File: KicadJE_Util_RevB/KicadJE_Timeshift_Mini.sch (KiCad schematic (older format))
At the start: 60 parts, among them J301 In3.1, J302 Out3.1, J303 Out3.2, P301 HEADER_2x5_Doepfer, U301 TL072, U302 TL072

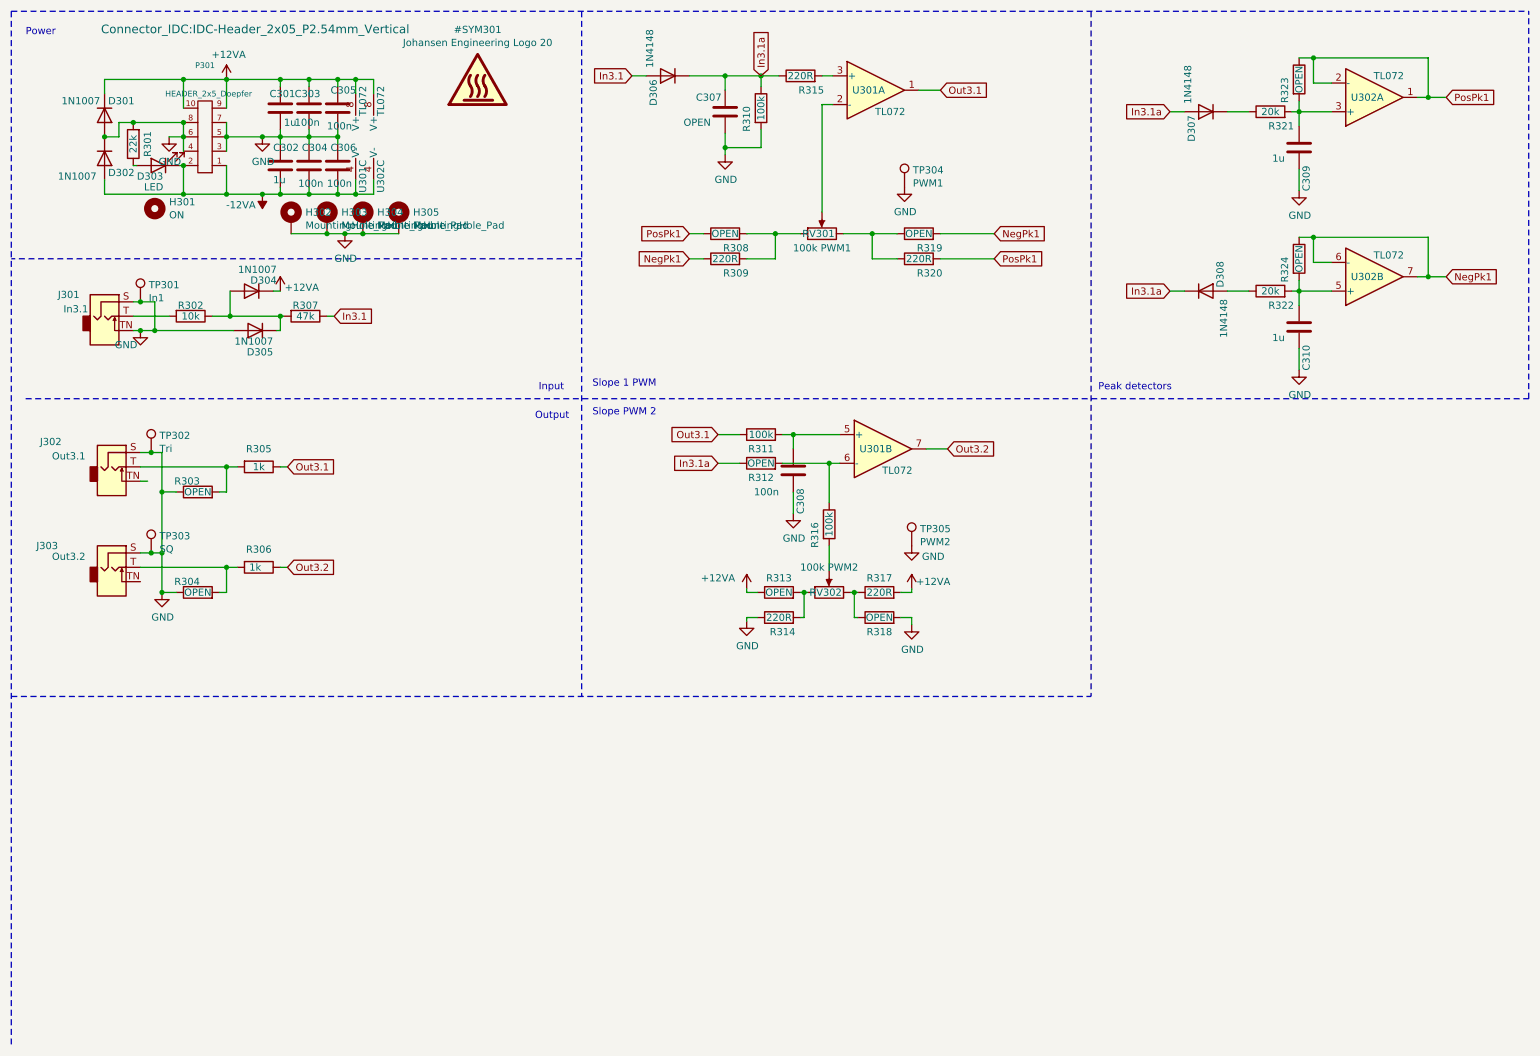
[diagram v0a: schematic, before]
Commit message: Update KicadJE_Timeshift_Mini.sch
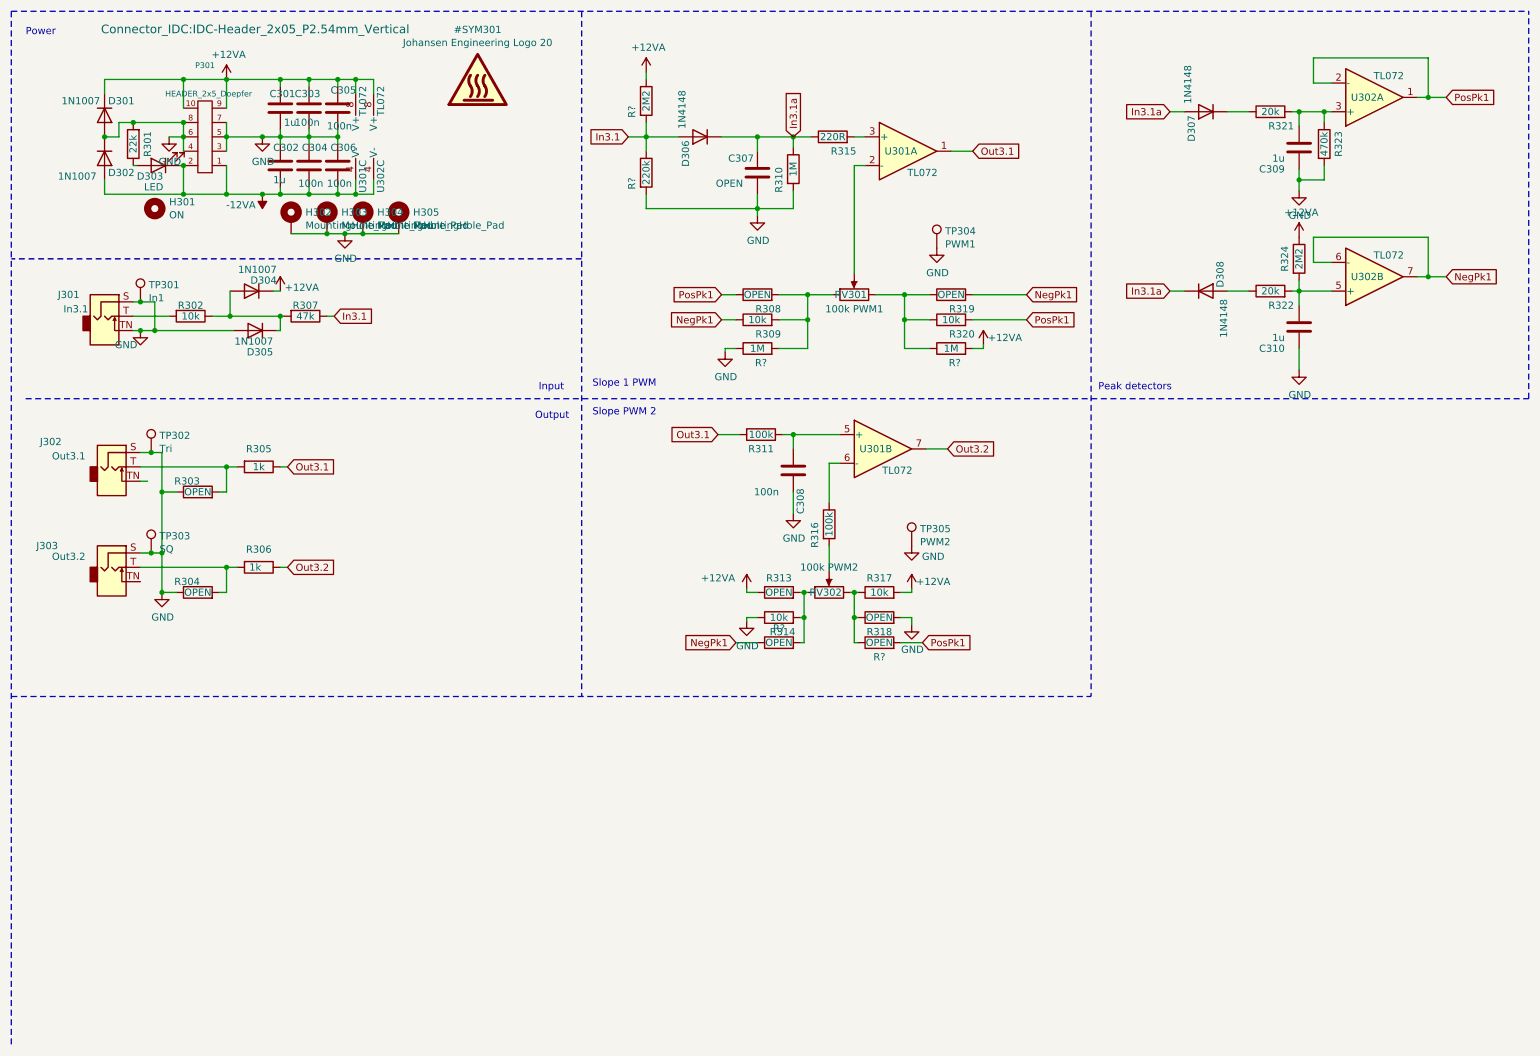
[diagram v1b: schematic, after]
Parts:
- removed R312: OPEN, Resistor_SMD:R_0805_2012Metric_Pad1.15x1.40mm_HandSolder, symbol Device:R
- added R?: 220k, Resistor_SMD:R_0805_2012Metric_Pad1.15x1.40mm_HandSolder, symbol Device:R
- added R?: 2M2, Resistor_SMD:R_0805_2012Metric_Pad1.15x1.40mm_HandSolder, symbol Device:R
- added R? (x2): 1M, Resistor_SMD:R_0805_2012Metric_Pad1.15x1.40mm_HandSolder, symbol Device:R
- added R? (x2): OPEN, Resistor_SMD:R_0805_2012Metric_Pad1.15x1.40mm_HandSolder, symbol Device:R
- R309, R314, R317, R320: value 220R -> 10k
- R310: value 100k -> 1M
- R323: value OPEN -> 470k
- R324: value OPEN -> 2M2
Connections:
- net +12VA: now also R324.1, R?.1, R?.2
- net GND: now also R323.2, R?.1, R?.2
- net In3.1: now also R?.1, R?.2
- net NegPk1: now also R?.1; no longer R324.1
- net PosPk1: now also R?.2; no longer R323.1
- net at R308.2, R309.2, RV301.1: now also R?.2
- net at R319.1, R320.1, RV301.3: now also R?.1
- net at C309.2, R321.2, U302.3 (+): now also R323.1; no longer R323.2
- net at R313.2, R314.2, RV302.1: now also R?.2
- net at R317.1, R318.1, RV302.3: now also R?.1
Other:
- moved on the sheet: C307, D306, R308, R309, R310, R315, R319, R320, R323, RV301, TP304, U301A

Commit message: Update KicadJE_Timeshift_Mini.sch
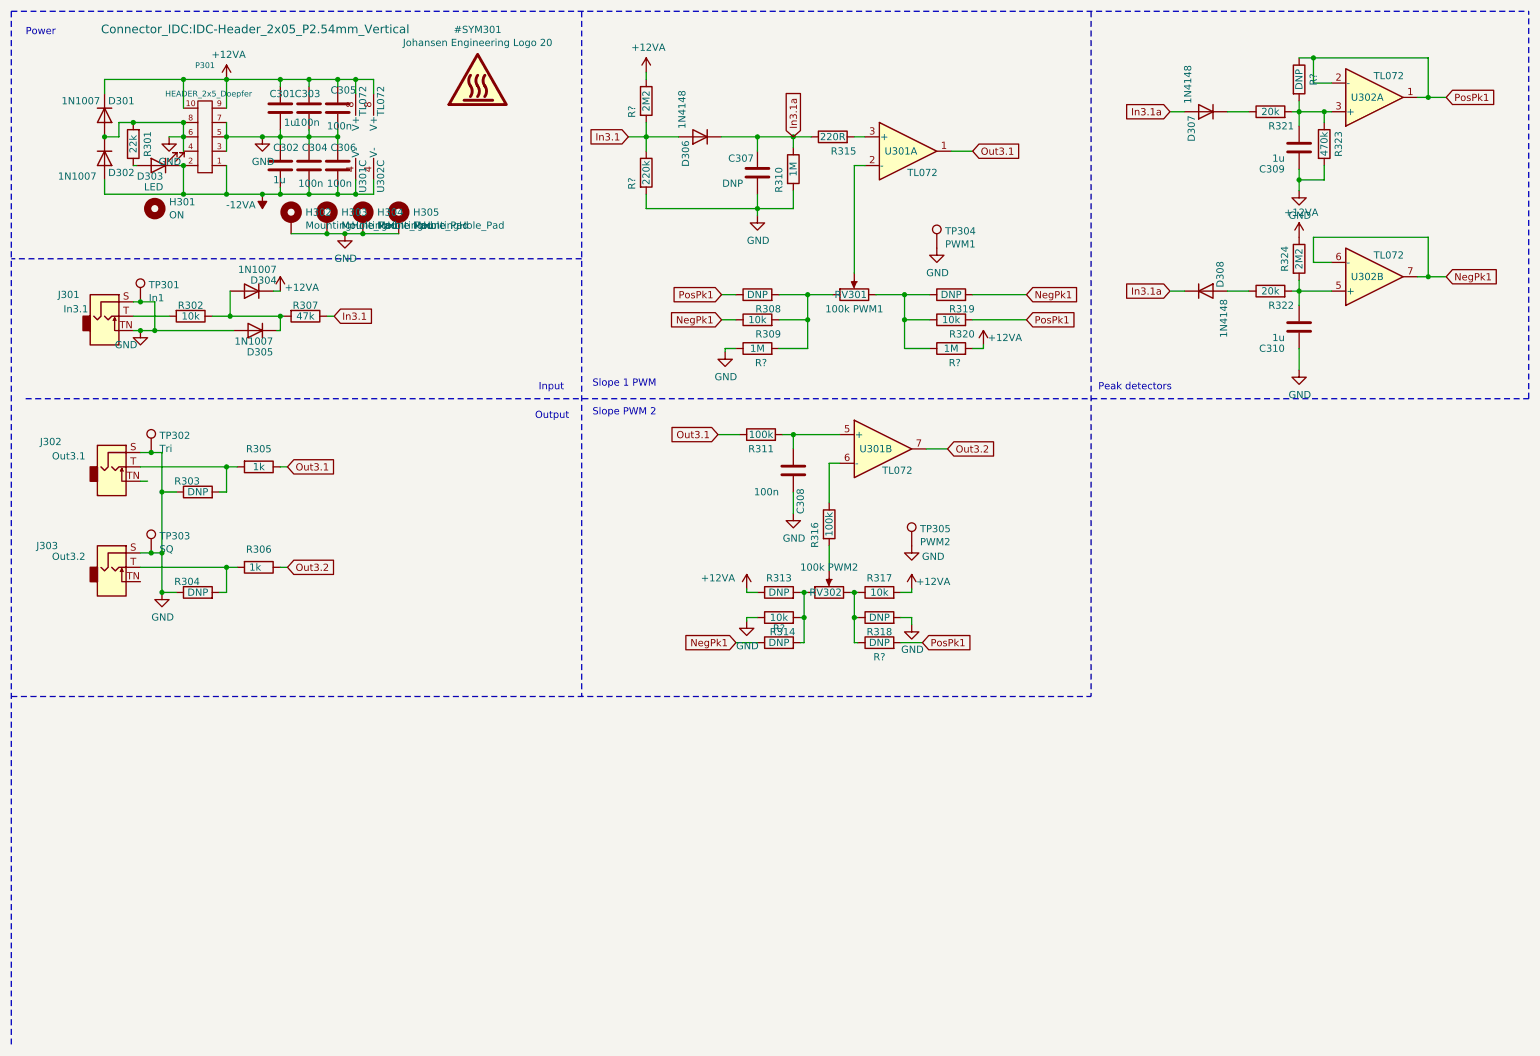
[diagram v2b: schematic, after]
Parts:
- added R?: DNP, Resistor_SMD:R_0805_2012Metric_Pad1.15x1.40mm_HandSolder, symbol Device:R
- C307, R303, R304, R308, R313, R318, R319, R? (x2): value OPEN -> DNP
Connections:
- net PosPk1: now also R?.1
- net at C309.2, R321.2, R323.1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: now also R?.2
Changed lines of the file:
@@
 AR Path="/5EFABE3E/5EFCD44F" Ref="R304"  Part="1"
 F 0 "R304" V 1900 4675 50  0000 C CNN
-F 1 "OPEN" V 1825 4600 50  0000 C CNN
+F 1 "DNP" V 1825 4600 50  0000 C CNN
 F 2 "Resistor_SMD:R_0805_2012Metric_Pad1.15x1.40mm_HandSolder" V 1755 4600 50  0001 C CNN
 F 3 "~" H 1825 4600 50  0001 C CNN
@@
 AR Path="/5EFABE3E/5EFCD52A" Ref="R303"  Part="1"
 F 0 "R303" V 1900 3975 50  0000 C CNN
-F 1 "OPEN" V 1825 3900 50  0000 C CNN
+F 1 "DNP" V 1825 3900 50  0000 C CNN
 F 2 "Resistor_SMD:R_0805_2012Metric_Pad1.15x1.40mm_HandSolder" V 1755 3900 50  0001 C CNN
 F 3 "~" H 1825 3900 50  0001 C CNN
@@
 AR Path="/5EFABE3E/5F001C3B" Ref="R308"  Part="1"
 F 0 "R308" V 5625 2450 50  0000 C CNN
-F 1 "OPEN" V 5725 2525 50  0000 C CNN
+F 1 "DNP" V 5725 2525 50  0000 C CNN
 F 2 "Resistor_SMD:R_0805_2012Metric_Pad1.15x1.40mm_HandSolder" V 5655 2525 50  0001 C CNN
 F 3 "~" H 5725 2525 50  0001 C CNN
@@
 AR Path="/5EFABE3E/5F001CA1" Ref="C307"  Part="1"
 F 0 "C307" H 5750 1575 50  0000 L CNN
-F 1 "OPEN" H 5825 1750 50  0000 L CNN
+F 1 "DNP" H 5825 1750 50  0000 L CNN
 F 2 "Capacitor_SMD:C_0805_2012Metric_Pad1.15x1.40mm_HandSolder" H 5763 1525 50  0001 C CNN
 F 3 "~" H 5725 1675 50  0001 C CNN
@@
 AR Path="/5EFABE3E/5F122A16" Ref="R319"  Part="1"
 F 0 "R319" V 6975 2450 50  0000 C CNN
-F 1 "OPEN" V 7075 2525 50  0000 C CNN
+F 1 "DNP" V 7075 2525 50  0000 C CNN
 F 2 "Resistor_SMD:R_0805_2012Metric_Pad1.15x1.40mm_HandSolder" V 7005 2525 50  0001 C CNN
 F 3 "~" H 7075 2525 50  0001 C CNN
@@
 AR Path="/5EFABE3E/5F1DE0C3" Ref="R313"  Part="1"
 F 0 "R313" V 5975 4600 50  0000 C CNN
-F 1 "OPEN" V 5875 4600 50  0000 C CNN
+F 1 "DNP" V 5875 4600 50  0000 C CNN
 F 2 "Resistor_SMD:R_0805_2012Metric_Pad1.15x1.40mm_HandSolder" V 5805 4600 50  0001 C CNN
 F 3 "~" H 5875 4600 50  0001 C CNN
@@
 AR Path="/5EFABE3E/5F1DE11A" Ref="R318"  Part="1"
 F 0 "R318" V 6475 4775 50  0000 C CNN
-F 1 "OPEN" V 6575 4775 50  0000 C CNN
+F 1 "DNP" V 6575 4775 50  0000 C CNN
 F 2 "Resistor_SMD:R_0805_2012Metric_Pad1.15x1.40mm_HandSolder" V 6505 4775 50  0001 C CNN
 F 3 "~" H 6575 4775 50  0001 C CNN
@@
 AR Path="/5EFABE3E/5EA9FF23" Ref="R?"  Part="1"
 F 0 "R?" V 6475 4950 50  0000 C CNN
-F 1 "OPEN" V 6575 4950 50  0000 C CNN
+F 1 "DNP" V 6575 4950 50  0000 C CNN
 F 2 "Resistor_SMD:R_0805_2012Metric_Pad1.15x1.40mm_HandSolder" V 6505 4950 50  0001 C CNN
 F 3 "~" H 6575 4950 50  0001 C CNN
@@
 AR Path="/5EFABE3E/5EAAADA4" Ref="R?"  Part="1"
 F 0 "R?" V 5975 4950 50  0000 C CNN
-F 1 "OPEN" V 5875 4950 50  0000 C CNN
+F 1 "DNP" V 5875 4950 50  0000 C CNN
 F 2 "Resistor_SMD:R_0805_2012Metric_Pad1.15x1.40mm_HandSolder" V 5805 4950 50  0001 C CNN
 F 3 "~" H 5875 4950 50  0001 C CNN
@@
 Wire Wire Line
 	5575 4950 5725 4950
+$Comp
+L Device:R R?
+U 1 1 5EB19454
+P 9500 1025
+AR Path="/5EB19454" Ref="R?"  Part="1"
+AR Path="/5C8C5FC0/5EB19454" Ref="R?"  Part="1"
+AR Path="/5CAAE8D3/5EB19454" Ref="R?"  Part="1"
+AR Path="/5E4B0DD9/5EB19454" Ref="R?"  Part="1"
+AR Path="/5E62ACA1/5EB19454" Ref="R?"  Part="1"
+AR Path="/5F49A670/5EB19454" Ref="R?"  Part="1"
+AR Path="/5FDBD837/5EB19454" Ref="R?"  Part="1"
+AR Path="/5EFABE3E/5EB19454" Ref="R?"  Part="1"
+F 0 "R?" V 9600 1025 50  0000 C CNN
+F 1 "DNP" V 9500 1025 50  0000 C CNN
+F 2 "Resistor_SMD:R_0805_2012Metric_Pad1.15x1.40mm_HandSolder" V 9430 1025 50  0001 C CNN
+F 3 "~" H 9500 1025 50  0001 C CNN
+	1    9500 1025
+	1    0    0    -1
+$EndComp
+Wire Wire Line
+	9500 1250 9500 1175
+Connection ~ 9600 875
+Wire Wire Line
+	9500 875  9600 875
 $EndSCHEMATC

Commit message: attempt to go to Kicad 7
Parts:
- P301: symbol Eurorack:HEADER_2x5_Doepfer -> KicadJE_Util-rescue:HEADER_2x5_Doepfer-Eurorack
- RV301, RV302: symbol Envelope-cache-2018-08-04-13-00-04:POT -> KicadJE_Util-rescue:POT-Envelope-cache-2018-08-04-13-00-04
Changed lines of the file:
@@
 $EndComp
 $Comp
-L Envelope-cache-2018-08-04-13-00-04:GND #PWR?
+L KicadJE_Util-rescue:GND-Envelope-cache-2018-08-04-13-00-04 #PWR?
 U 1 1 5EFCD382
 P 1575 4600
@@
 $EndComp
 $Comp
-L Eurorack:HEADER_2x5_Doepfer P?
+L KicadJE_Util-rescue:HEADER_2x5_Doepfer-Eurorack P?
 U 1 1 5EFCD3D2
 P 1875 1425
@@
 	2400 1075 2400 1025
 $Comp
-L Envelope-cache-2018-08-04-13-00-04:GND #PWR?
+L KicadJE_Util-rescue:GND-Envelope-cache-2018-08-04-13-00-04 #PWR?
 U 1 1 5EFCD408
 P 2275 1425
@@
 $EndComp
 $Comp
-L Envelope-cache-2018-08-04-13-00-04:GND #PWR?
+L KicadJE_Util-rescue:GND-Envelope-cache-2018-08-04-13-00-04 #PWR?
 U 1 1 5EFCD41A
 P 1625 1425
@@
 Connection ~ 2975 2100
 $Comp
-L Envelope-cache-2018-08-04-13-00-04:GND #PWR?
+L KicadJE_Util-rescue:GND-Envelope-cache-2018-08-04-13-00-04 #PWR?
 U 1 1 5EFCD514
 P 2850 2100
@@
 	1425 2575 1375 2575
 $Comp
-L Envelope-cache-2018-08-04-13-00-04:GND #PWR?
+L KicadJE_Util-rescue:GND-Envelope-cache-2018-08-04-13-00-04 #PWR?
 U 1 1 5F001BB2
 P 1425 2775
@@
 $EndComp
 $Comp
-L Envelope-cache-2018-08-04-13-00-04:POT RV?
+L KicadJE_Util-rescue:POT-Envelope-cache-2018-08-04-13-00-04 RV?
 U 1 1 5F001C35
 P 6400 2525
@@
 $EndComp
 $Comp
-L Envelope-cache-2018-08-04-13-00-04:GND #PWR?
+L KicadJE_Util-rescue:GND-Envelope-cache-2018-08-04-13-00-04 #PWR?
 U 1 1 5F001C50
 P 6975 2200
@@
 	5575 2525 5475 2525
 $Comp
-L Envelope-cache-2018-08-04-13-00-04:GND #PWR?
+L KicadJE_Util-rescue:GND-Envelope-cache-2018-08-04-13-00-04 #PWR?
 U 1 1 5F001C8C
 P 5725 1975
@@
 	7225 2700 7600 2700
 $Comp
-L Envelope-cache-2018-08-04-13-00-04:GND #PWR?
+L KicadJE_Util-rescue:GND-Envelope-cache-2018-08-04-13-00-04 #PWR?
 U 1 1 5F1554B9
 P 9500 1800
@@
 $EndComp
 $Comp
-L Envelope-cache-2018-08-04-13-00-04:GND #PWR?
+L KicadJE_Util-rescue:GND-Envelope-cache-2018-08-04-13-00-04 #PWR?
 U 1 1 5F1A0D96
 P 9500 3050
@@
 $EndComp
 $Comp
-L Envelope-cache-2018-08-04-13-00-04:POT RV?
+L KicadJE_Util-rescue:POT-Envelope-cache-2018-08-04-13-00-04 RV?
 U 1 1 5F1DE0B9
 P 6225 4600
@@
 $EndComp
 $Comp
-L Envelope-cache-2018-08-04-13-00-04:GND #PWR?
+L KicadJE_Util-rescue:GND-Envelope-cache-2018-08-04-13-00-04 #PWR?
 U 1 1 5F1DE0D7
 P 6800 4275
@@
 $EndComp
 $Comp
-L Envelope-cache-2018-08-04-13-00-04:GND #PWR?
+L KicadJE_Util-rescue:GND-Envelope-cache-2018-08-04-13-00-04 #PWR?
 U 1 1 5F1DE0E2
 P 5975 4050
@@
 	5975 3900 5975 4050
 $Comp
-L Envelope-cache-2018-08-04-13-00-04:GND #PWR?
+L KicadJE_Util-rescue:GND-Envelope-cache-2018-08-04-13-00-04 #PWR?
 U 1 1 5F297E88
 P 6800 4825
@@
 $EndComp
 $Comp
-L Envelope-cache-2018-08-04-13-00-04:GND #PWR?
+L KicadJE_Util-rescue:GND-Envelope-cache-2018-08-04-13-00-04 #PWR?
 U 1 1 5F297754
 P 5650 4800
@@
 $EndComp
 $Comp
-L Envelope-cache-2018-08-04-13-00-04:GND #PWR?
+L KicadJE_Util-rescue:GND-Envelope-cache-2018-08-04-13-00-04 #PWR?
 U 1 1 5EA79FA1
 P 5500 2925
